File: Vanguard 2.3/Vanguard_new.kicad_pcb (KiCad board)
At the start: 4 copper layers, 42.3 x 51.9 mm, 88 parts, among them J1 USB_C_Receptacle_USB2.0_16P, J2 Conn_02x03_Pin, J3 Micro_SD_Card_Det1, J4 STARBOARD_SERVO, J5 PORTSIDE_SERVO, J6 Battery In, J7 EJECTION_SERVO, Q1 BSS138, Q2 BSS138, Q3 BSS138, Q4 BSS138, U1 ATSAMD11D14A-M, U2 ATmega4809-A, U3 AT25DF641A-SH-T, U4 AP2112K-3.3, U5 BD1020HFV, U6 BNO086, U7 TXB0104D, U8 TPS61092, U9 MPM3610AGQV-P, Y1 32.768kHz

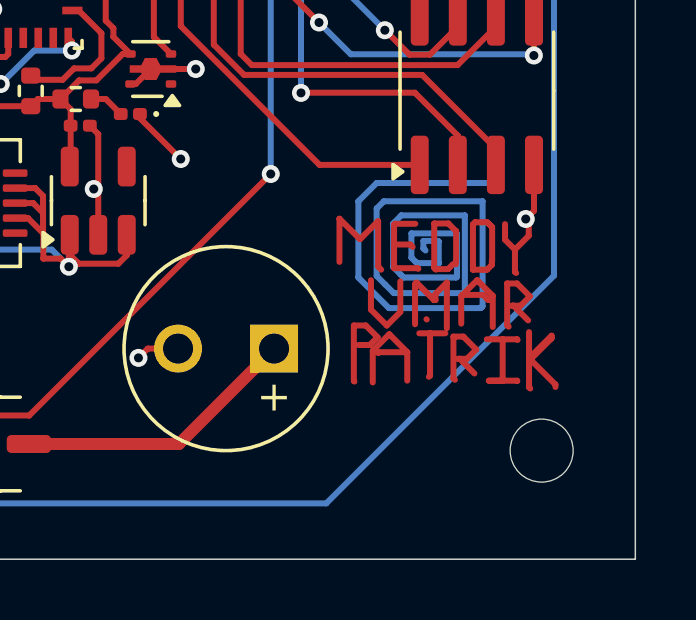
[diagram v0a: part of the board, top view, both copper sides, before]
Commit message: i forgot what i did
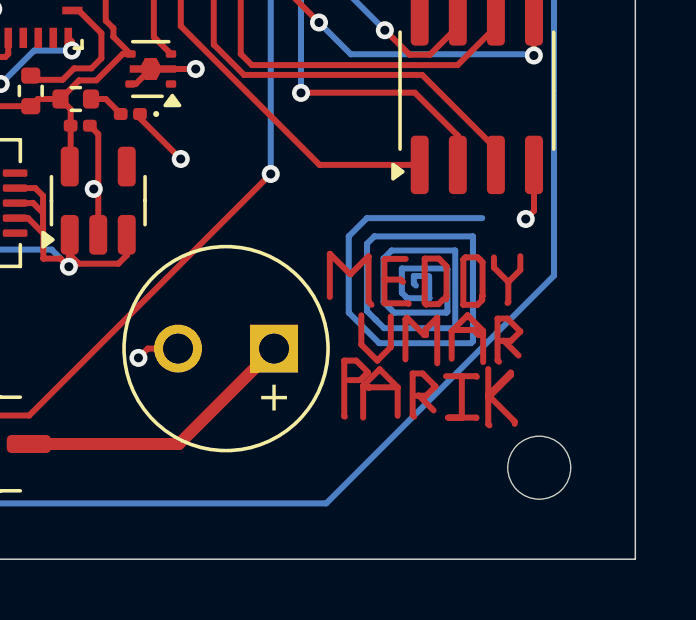
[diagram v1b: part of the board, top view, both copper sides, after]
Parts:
- moved REF** 0.58 mm to (131.4, 132.8)
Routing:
- net GND: track 69.1 -> 66.3 mm
